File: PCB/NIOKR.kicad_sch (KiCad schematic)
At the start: 47 parts

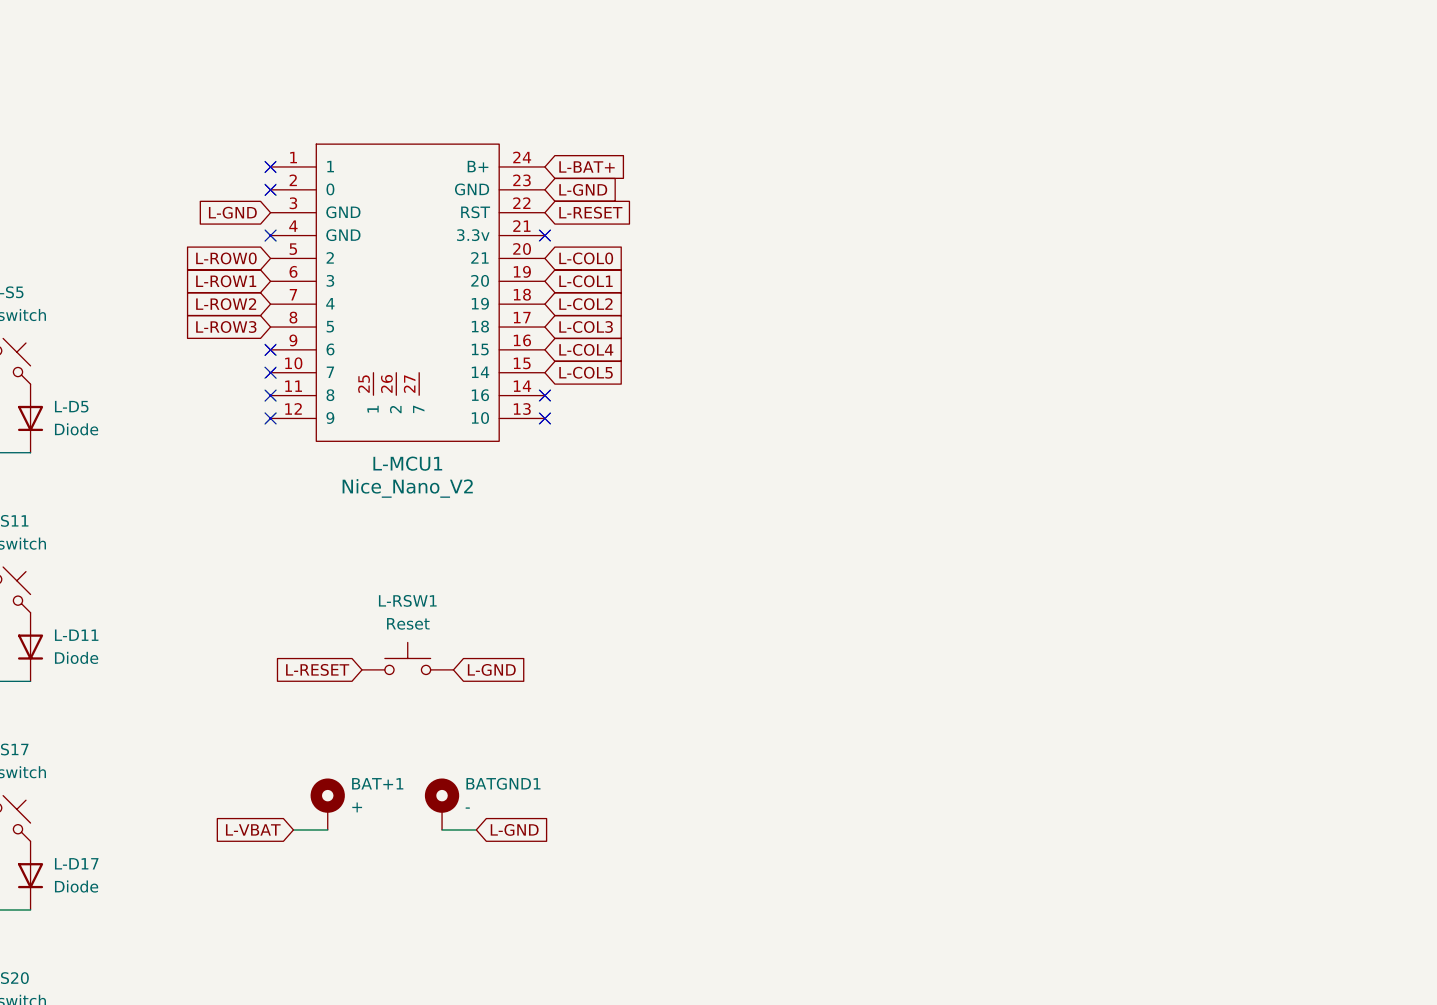
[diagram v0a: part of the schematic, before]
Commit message: houdini routing
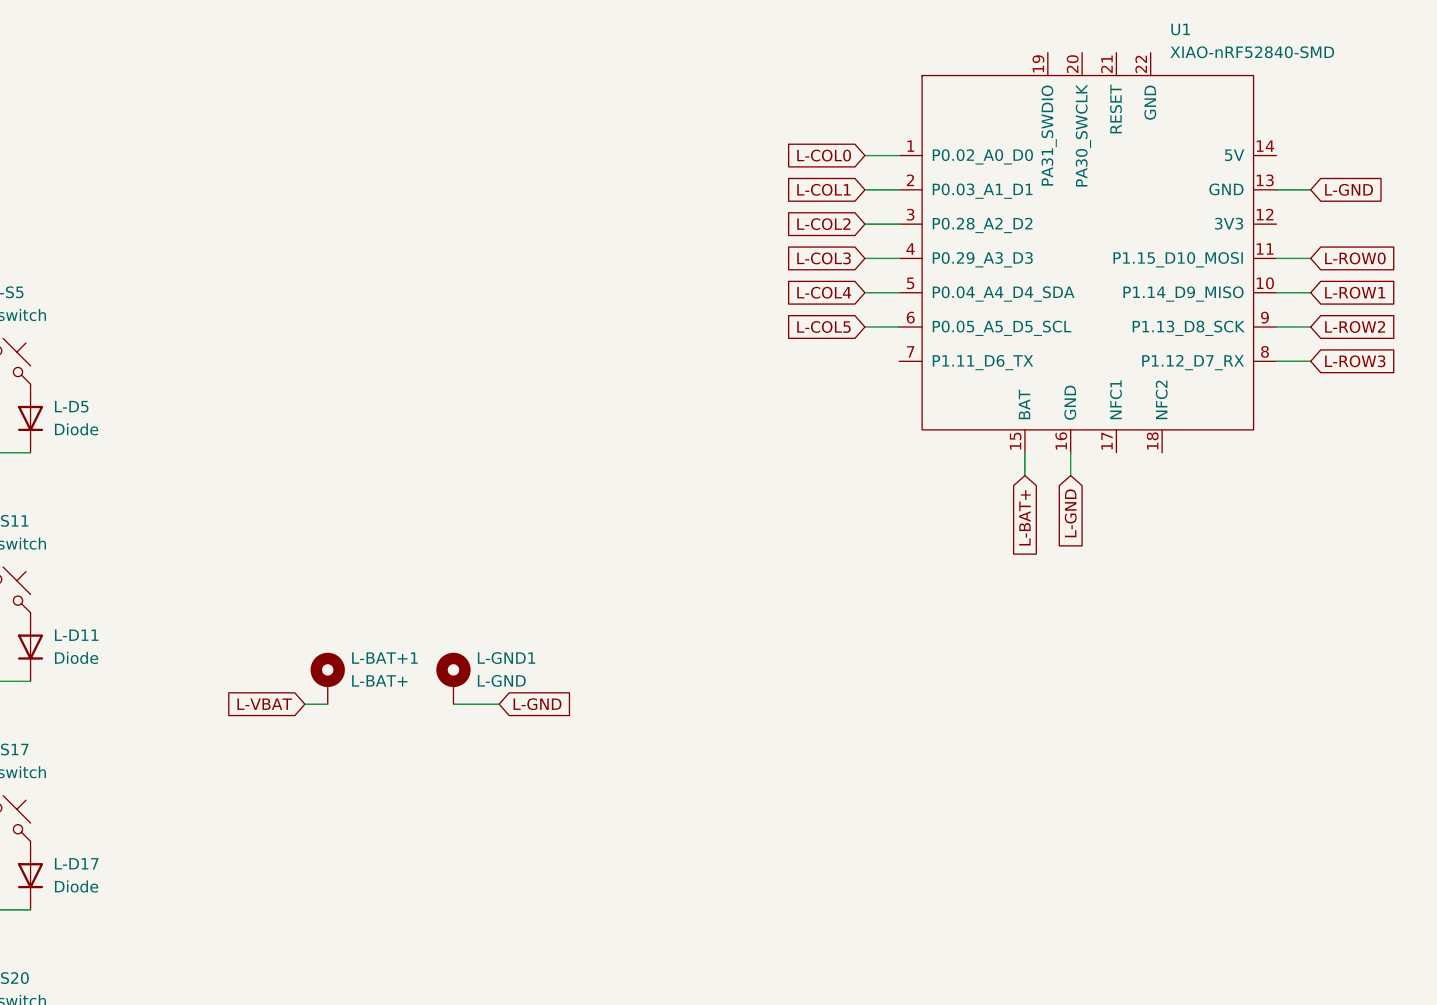
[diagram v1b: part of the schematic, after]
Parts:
- removed BAT+1: +, TOTEMlib:BatteryPad, symbol Mechanical:MountingHole_Pad_MP
- removed BATGND1: -, TOTEMlib:BatteryPad, symbol Mechanical:MountingHole_Pad_MP
- removed L-MCU1: Nice_Nano_V2, MCU:Nice_Nano_V2, symbol NIOKR_symbols:MCU_Nice_Nano_V2
- removed L-RSW1: Reset, TOTEMlib:SKHLLCA010, symbol NIOKR_symbols:Placeholder_Switch
- added L-BAT+1: L-BAT+, TOTEMlib:BatteryPad, symbol Mechanical:MountingHole_Pad_MP
- added L-GND1: L-GND, TOTEMlib:BatteryPad, symbol Mechanical:MountingHole_Pad_MP
- added U1: XIAO-nRF52840-SMD, Seeed Studio XIAO Series Library:XIAO-nRF52840-SMD, symbol Seeed_Studio_XIAO_Series:XIAO-nRF52840-SMD
- L-S0, L-S1, L-S2, L-S3, L-S4, L-S5: footprint Hotswap:Hotswap_Choc_V1V2_neri_klp_saddle_tilted_top -> Hotswap:Hotswap_Choc_V1V2_klp_saddle
- L-S10: footprint Hotswap:Hotswap_Choc_V1V2_klp_saddle_homing -> Hotswap:Hotswap_Choc_V1V2_klp_saddle
- L-S12, L-S13, L-S14, L-S15, L-S16, L-S17: footprint Hotswap:Hotswap_Choc_V1V2_neri_klp_saddle_tilted_bottom -> Hotswap:Hotswap_Choc_V1V2_klp_saddle
- L-S18, L-S19, L-S20: footprint Hotswap:Hotswap_Choc_V1V2_neri_klp_saddle_thumb -> Hotswap:Hotswap_Choc_V1V2_klp_saddle
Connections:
- net L-BAT+: now also U1.15 (BAT)
- net L-COL0: now also U1.1 (P0.02_A0_D0)
- net L-COL1: now also U1.2 (P0.03_A1_D1)
- net L-COL2: now also U1.3 (P0.28_A2_D2)
- net L-COL3: now also U1.4 (P0.29_A3_D3)
- net L-COL4: now also U1.5 (P0.04_A4_D4_SDA)
- net L-COL5: now also U1.6 (P0.05_A5_D5_SCL)
- net L-GND: now also L-GND1.1 (GND), U1.13 (GND), U1.16 (GND)
- net L-ROW0: now also U1.11 (P1.15_D10_MOSI)
- net L-ROW1: now also U1.10 (P1.14_D9_MISO)
- net L-ROW2: now also U1.9 (P1.13_D8_SCK)
- net L-ROW3: now also U1.8 (P1.12_D7_RX)
- net L-VBAT: now also L-BAT+1.1 (BAT+)
- no-connect marks 11 -> 1

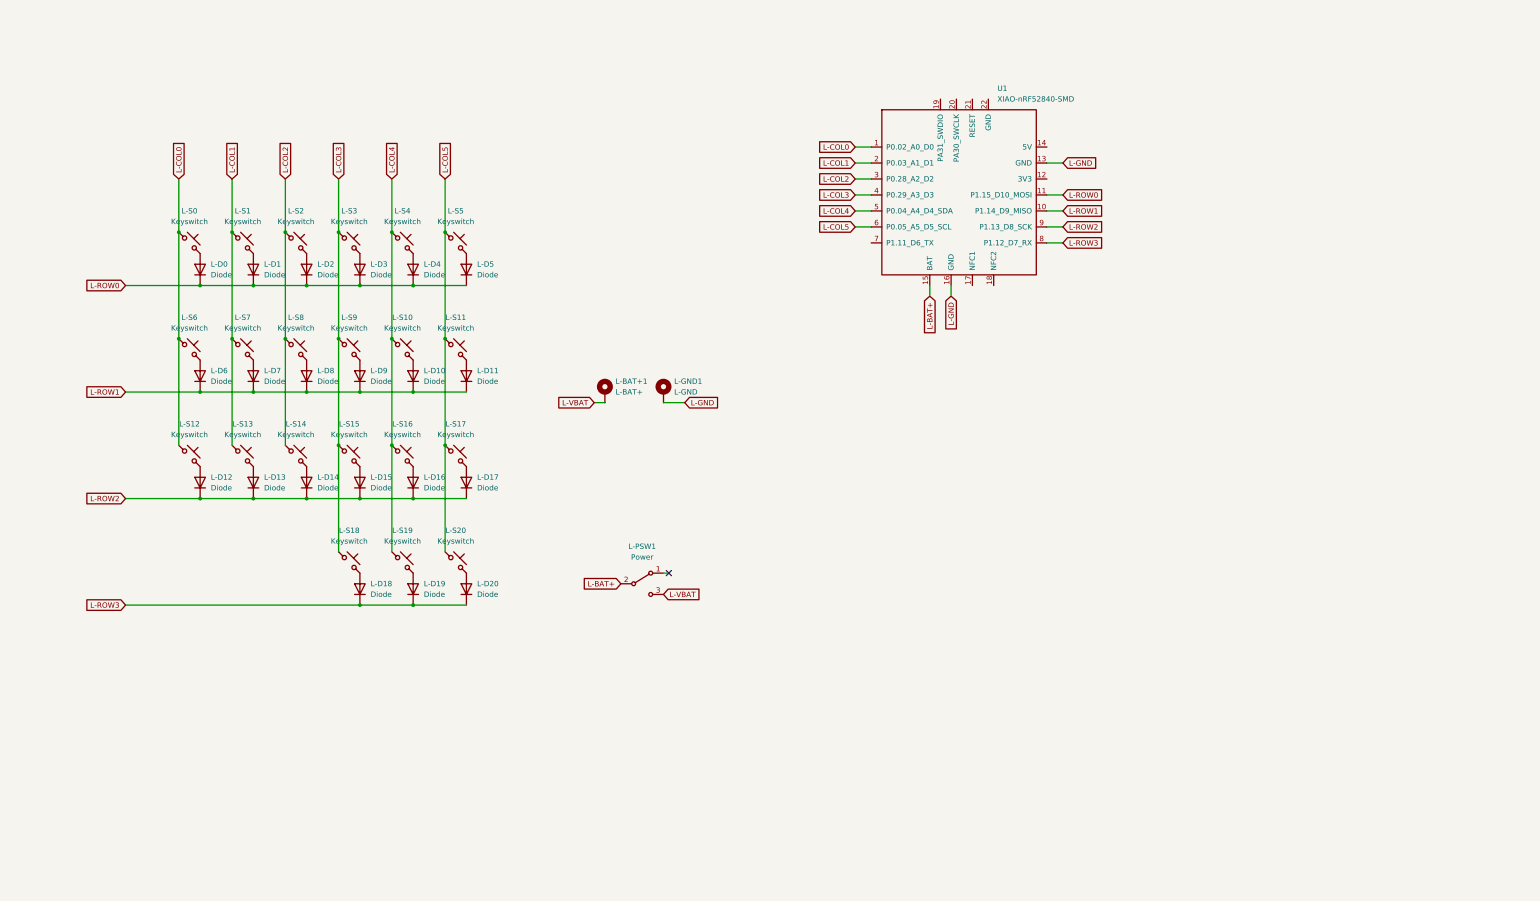
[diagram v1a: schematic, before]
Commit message: current
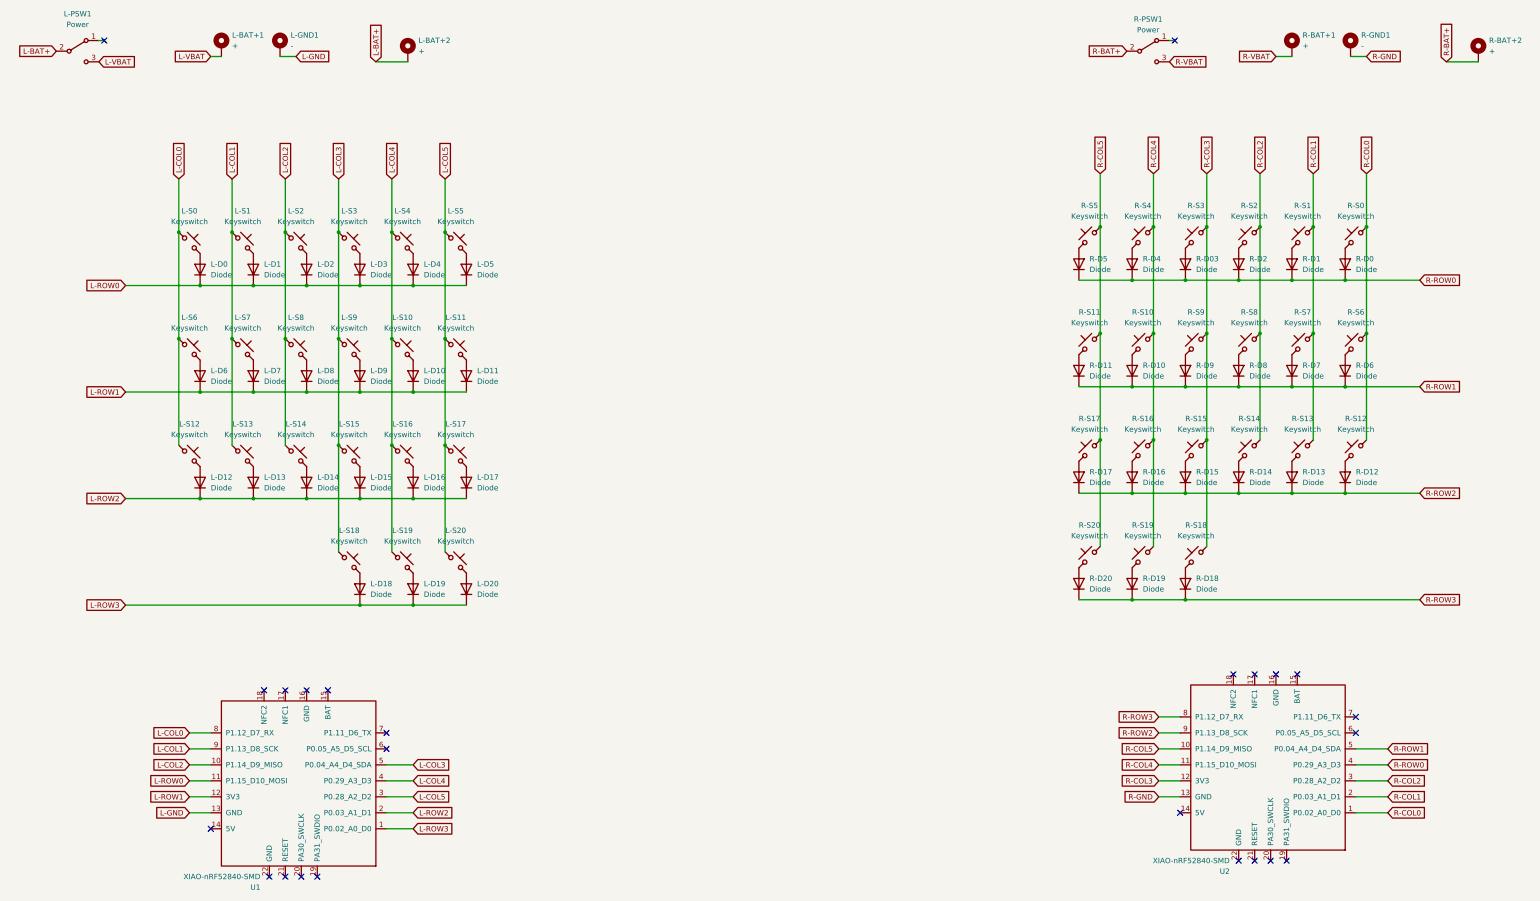
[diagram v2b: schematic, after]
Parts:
- added L-BAT+2, R-BAT+1, R-BAT+2: +, NII:BatteryPad, symbol Mechanical:MountingHole_Pad_MP
- added R-D0, R-D03, R-D1, R-D10, R-D11, R-D12, R-D13, R-D14, R-D15, R-D16, R-D17, R-D18, R-D19, R-D2, R-D20, R-D4, R-D5, R-D6, R-D7, R-D8, R-D9: Diode, NII:Diode_SOD123, symbol NIOKR_symbols:Placeholder_Diode
- added R-GND1: -, NII:BatteryPad, symbol Mechanical:MountingHole_Pad_MP
- added R-PSW1: Power, NII:MSK12C02, symbol Switch:SW_SPDT
- added R-S0, R-S1, R-S10, R-S11, R-S12, R-S13, R-S14, R-S15, R-S16, R-S17, R-S18, R-S19, R-S2, R-S20, R-S3, R-S4, R-S5, R-S6, R-S7, R-S8, R-S9: Keyswitch, NII:keyswitch_choc12_gateron_low_profile_hotswap_1u_no_led, symbol NIOKR_symbols:Placeholder_Keyswitch
- added U2: XIAO-nRF52840-SMD, NII:XIAO-nRF52840-cutout, symbol Seeed_Studio_XIAO_Series:XIAO-nRF52840-SMD
- L-BAT+1: value L-BAT+ -> +; footprint TOTEMlib:BatteryPad -> NII:BatteryPad
- L-D0, L-D1, L-D10, L-D11, L-D12, L-D13, L-D14, L-D15, L-D16, L-D17, L-D18, L-D19, L-D2, L-D20, L-D3, L-D4, L-D5, L-D6, L-D7, L-D8, L-D9: footprint Diode_SMD:D_SOD-123 -> NII:Diode_SOD123
- L-GND1: value L-GND -> -; footprint TOTEMlib:BatteryPad -> NII:BatteryPad
- L-PSW1: footprint TOTEMlib:MSK12C02 -> NII:MSK12C02
- L-S0, L-S1, L-S10, L-S11, L-S12, L-S13, L-S14, L-S15, L-S16, L-S17, L-S18, L-S19, L-S2, L-S20, L-S3, L-S4, L-S5, L-S6, L-S7, L-S8, L-S9: footprint Hotswap:Hotswap_Choc_V1V2_klp_saddle -> NII:keyswitch_choc12_gateron_low_profile_hotswap_1u_no_led
- U1: footprint Seeed Studio XIAO Series Library:XIAO-nRF52840-SMD -> NII:XIAO-nRF52840-cutout
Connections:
- net L-BAT+: now also L-BAT+2.1 (BAT+); no longer U1.15 (BAT)
- net L-COL0: now also U1.8 (P1.12_D7_RX); no longer U1.1 (P0.02_A0_D0)
- net L-COL1: now also U1.9 (P1.13_D8_SCK); no longer U1.2 (P0.03_A1_D1)
- net L-COL2: now also U1.10 (P1.14_D9_MISO); no longer U1.3 (P0.28_A2_D2)
- net L-COL3: now also U1.5 (P0.04_A4_D4_SDA); no longer U1.4 (P0.29_A3_D3)
- net L-COL4: now also U1.4 (P0.29_A3_D3); no longer U1.5 (P0.04_A4_D4_SDA)
- net L-COL5: now also U1.3 (P0.28_A2_D2); no longer U1.6 (P0.05_A5_D5_SCL)
- net L-GND: no longer U1.16 (GND)
- net L-ROW1: now also U1.12 (3V3); no longer U1.10 (P1.14_D9_MISO)
- net L-ROW2: now also U1.2 (P0.03_A1_D1); no longer U1.9 (P1.13_D8_SCK)
- net L-ROW3: now also U1.1 (P0.02_A0_D0); no longer U1.8 (P1.12_D7_RX)
- new net: R-D12.2 (A), R-S12.2
- new net: R-D11.2 (A), R-S11.2
- new net: R-D18.2 (A), R-S18.2
- new net: R-D6.2 (A), R-S6.2
- new net: R-D9.2 (A), R-S9.2
- new net: R-D10.2 (A), R-S10.2
- new net: R-D03.2 (A), R-S3.2
- new net: R-D17.2 (A), R-S17.2
- new net: R-D8.2 (A), R-S8.2
- new net: R-D0.2 (A), R-S0.2
- new net: R-D5.2 (A), R-S5.2
- new net: R-D20.2 (A), R-S20.2
- new net: R-D2.2 (A), R-S2.2
- new net: R-D4.2 (A), R-S4.2
- new net: R-D19.2 (A), R-S19.2
- new net: R-D16.2 (A), R-S16.2
- new net: R-D13.2 (A), R-S13.2
- new net: R-D1.2 (A), R-S1.2
- new net: R-D7.2 (A), R-S7.2
- new net: R-D14.2 (A), R-S14.2
- new net: R-D15.2 (A), R-S15.2
- new net R-BAT+: R-BAT+2.1 (BAT+), R-PSW1.2 (B)
- new net R-COL0: R-S0.1, R-S12.1, R-S6.1, U2.1 (P0.02_A0_D0)
- new net R-COL1: R-S1.1, R-S13.1, R-S7.1, U2.2 (P0.03_A1_D1)
- new net R-COL2: R-S14.1, R-S2.1, R-S8.1, U2.3 (P0.28_A2_D2)
- new net R-COL3: R-S15.1, R-S18.1, R-S3.1, R-S9.1, U2.12 (3V3)
- new net R-COL4: R-S10.1, R-S16.1, R-S19.1, R-S4.1, U2.11 (P1.15_D10_MOSI)
- new net R-COL5: R-S11.1, R-S17.1, R-S20.1, R-S5.1, U2.10 (P1.14_D9_MISO)
- new net R-GND: R-GND1.1 (GND), U2.13 (GND)
- new net R-ROW0: R-D0.1 (K), R-D03.1 (K), R-D1.1 (K), R-D2.1 (K), R-D4.1 (K), R-D5.1 (K), U2.4 (P0.29_A3_D3)
- new net R-ROW1: R-D10.1 (K), R-D11.1 (K), R-D6.1 (K), R-D7.1 (K), R-D8.1 (K), R-D9.1 (K), U2.5 (P0.04_A4_D4_SDA)
- new net R-ROW2: R-D12.1 (K), R-D13.1 (K), R-D14.1 (K), R-D15.1 (K), R-D16.1 (K), R-D17.1 (K), U2.9 (P1.13_D8_SCK)
- new net R-ROW3: R-D18.1 (K), R-D19.1 (K), R-D20.1 (K), U2.8 (P1.12_D7_RX)
- new net R-VBAT: R-BAT+1.1 (BAT+), R-PSW1.3 (C)
- no-connect marks 1 -> 24
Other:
- moved on the sheet: L-BAT+1, L-GND1, L-PSW1, U1
